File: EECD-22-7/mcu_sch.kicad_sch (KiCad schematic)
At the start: 10 parts, among them SW1 SW_Push, U1 STM32F103CBUx

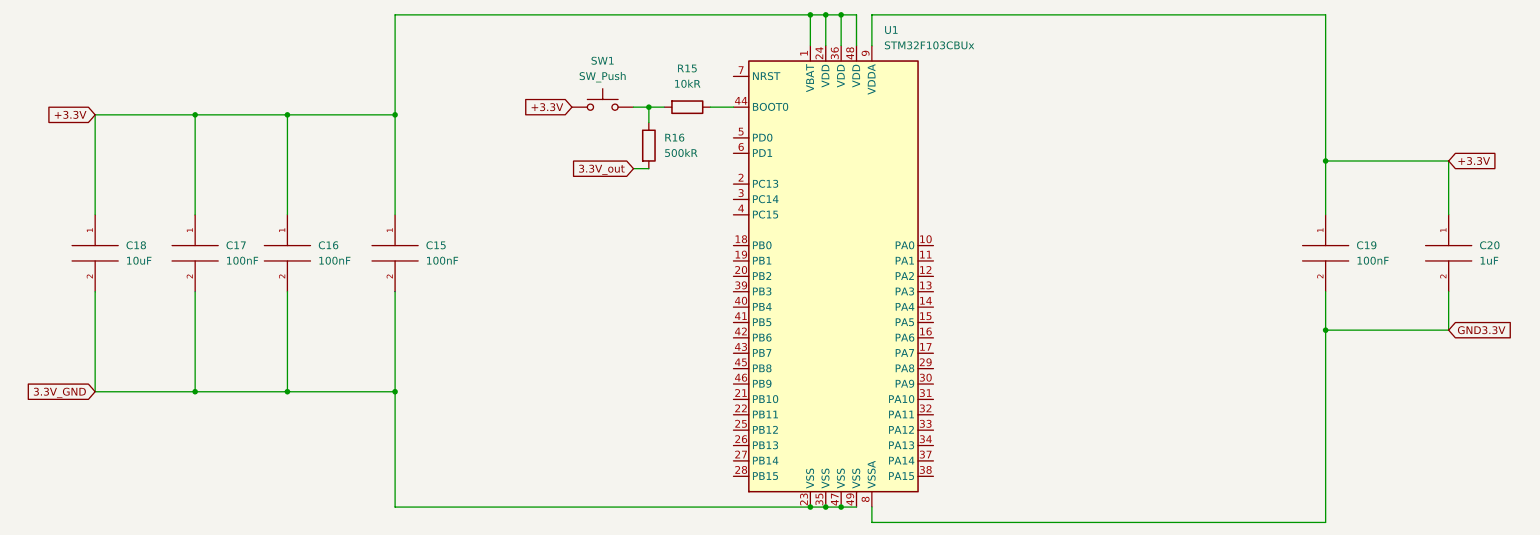
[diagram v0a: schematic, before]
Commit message: Add files via upload
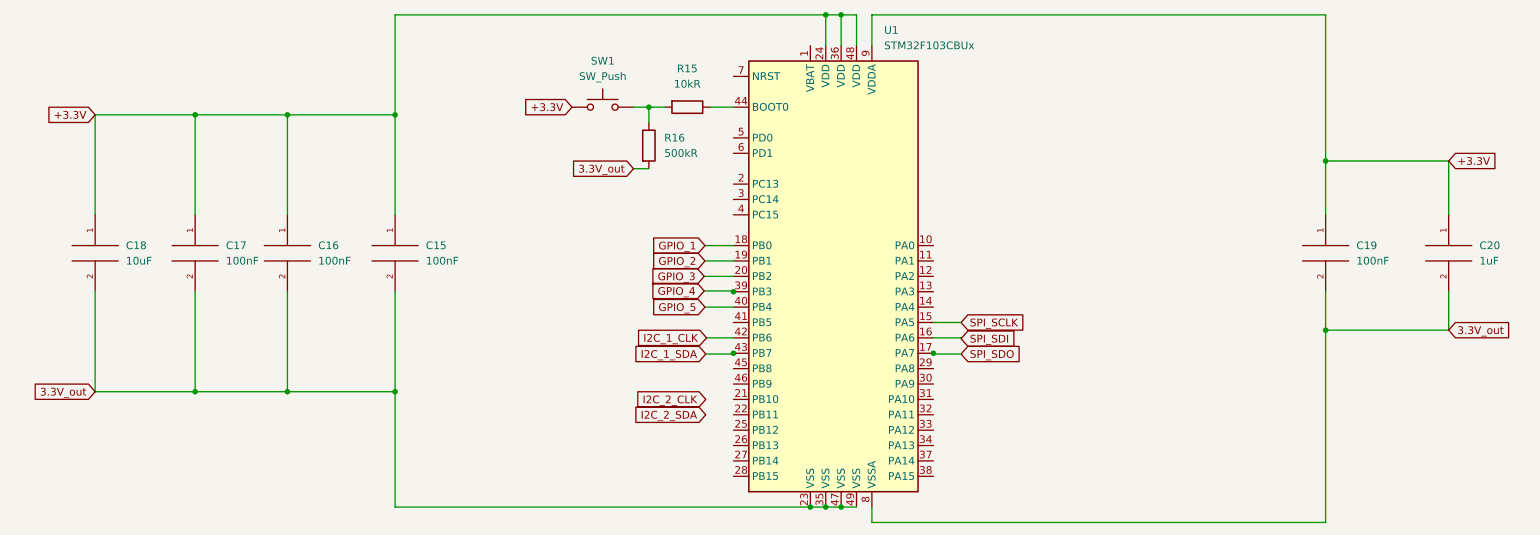
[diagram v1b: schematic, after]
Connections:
- net 3.3V_GND is gone; now on net 3.3V_out: C15.2, C16.2, C17.2, C18.2, U1.23 (VSS), U1.35 (VSS), U1.47 (VSS), U1.49 (VSS)
- net GND3.3V is gone; now on net 3.3V_out: C19.2, C20.2, U1.8 (VSSA)
- net +3.3V: no longer U1.1 (VBAT)
- net SPI_SCLK: now reaches U1.15 (PA5)
- net SPI_SDI: now reaches U1.16 (PA6)
- net SPI_SDO: now reaches U1.17 (PA7)
- net GPIO_1: now reaches U1.18 (PB0)
- net GPIO_2: now reaches U1.19 (PB1)
- net GPIO_3: now reaches U1.20 (PB2)
- net GPIO_4: now reaches U1.39 (PB3)
- net GPIO_5: now reaches U1.40 (PB4)
- net I2C_1_CLK: now reaches U1.42 (PB6)
- net I2C_1_SDA: now reaches U1.43 (PB7)

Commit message: Add files via upload
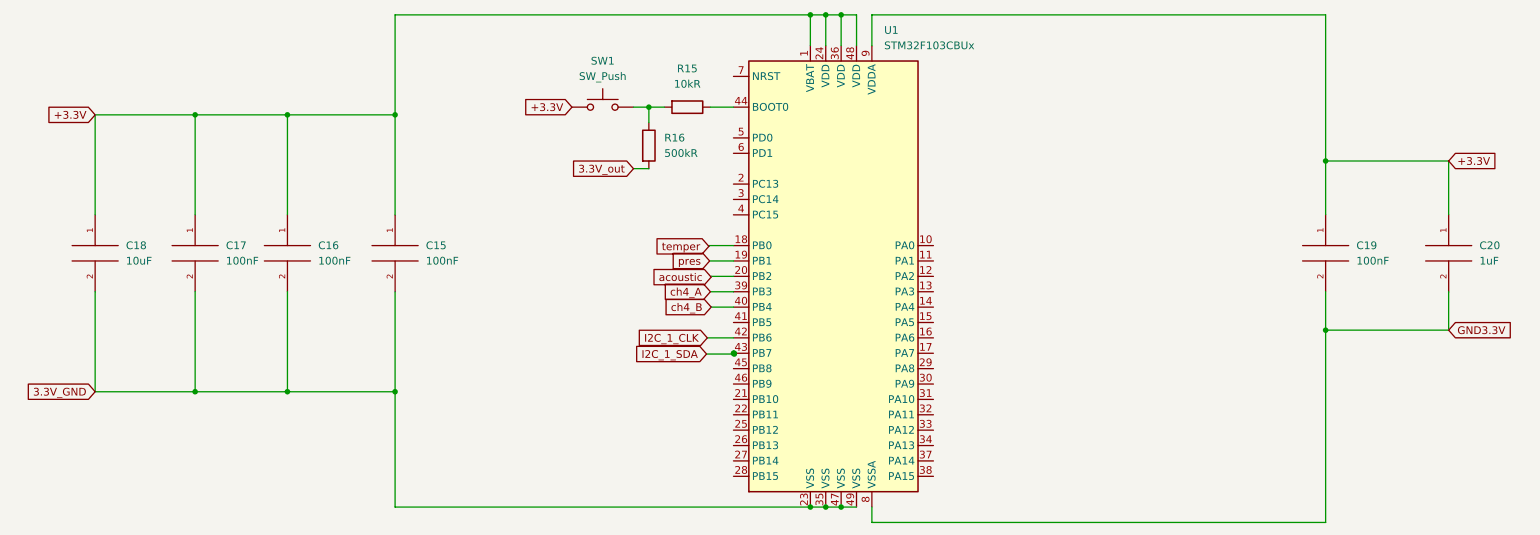
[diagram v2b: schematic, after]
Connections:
- net +3.3V: now also U1.1 (VBAT)
- net 3.3V_out: no longer C15.2, C16.2, C17.2, C18.2, C19.2, C20.2, U1.23 (VSS), U1.35 (VSS), U1.47 (VSS), U1.49 (VSS), U1.8 (VSSA)
- net GPIO_1 renamed temper
- net GPIO_2 renamed pres
- net GPIO_3 renamed acoustic
- net GPIO_4 renamed ch4_A
- net GPIO_5 renamed ch4_B
- net SPI_SCLK: no longer names the net of U1.15 (PA5)
- net SPI_SDI: no longer names the net of U1.16 (PA6)
- net SPI_SDO: no longer names the net of U1.17 (PA7)
- new net 3.3V_GND: C15.2, C16.2, C17.2, C18.2, U1.23 (VSS), U1.35 (VSS), U1.47 (VSS), U1.49 (VSS)
- new net GND3.3V: C19.2, C20.2, U1.8 (VSSA)
